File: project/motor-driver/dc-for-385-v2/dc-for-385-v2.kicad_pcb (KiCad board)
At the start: 2 copper layers, 51 x 25 mm, 44 parts, among them J1 Power, J2 Output, J3 Input, Q1 TPH11006NL, Q2 TPH11006NL, Q3 TPH11006NL, Q4 TPH11006NL, U1 IR2302, U2 IR2302, U3 L7808

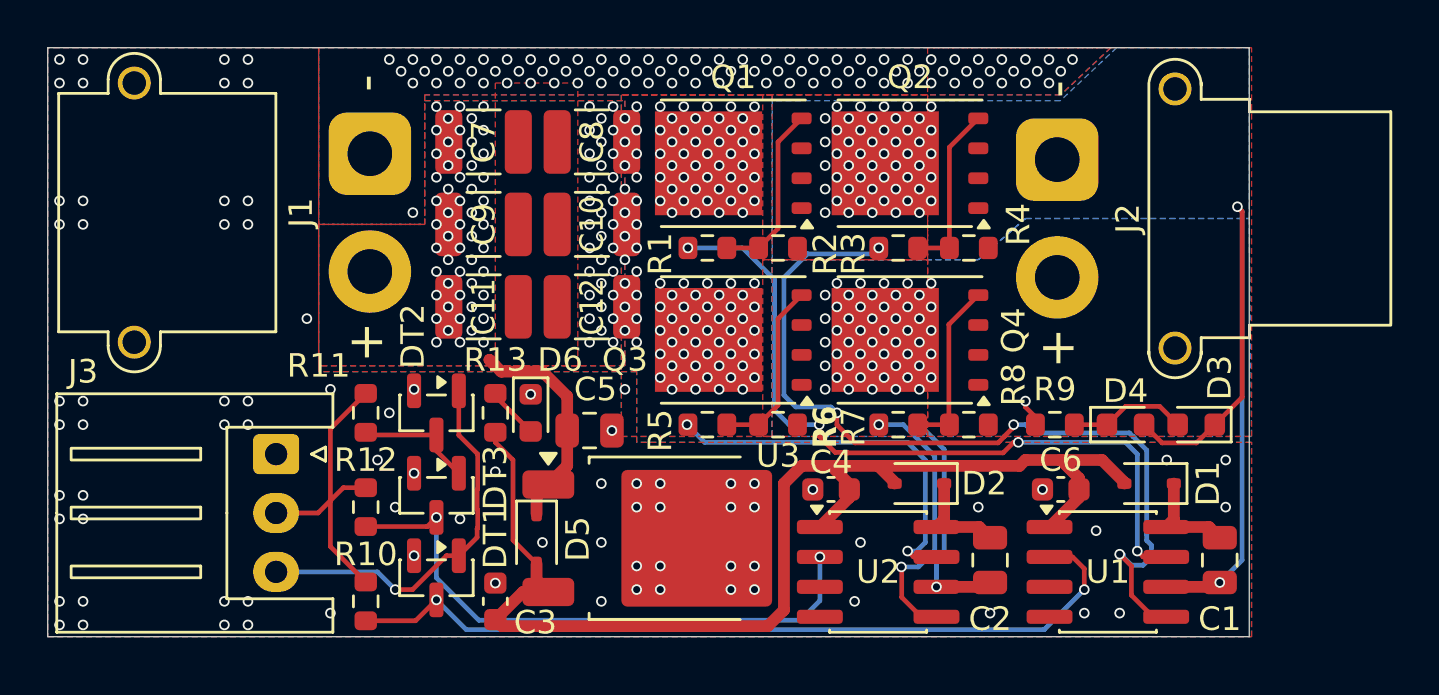
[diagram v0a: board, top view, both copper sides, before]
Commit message: 2026/07/07/11:00
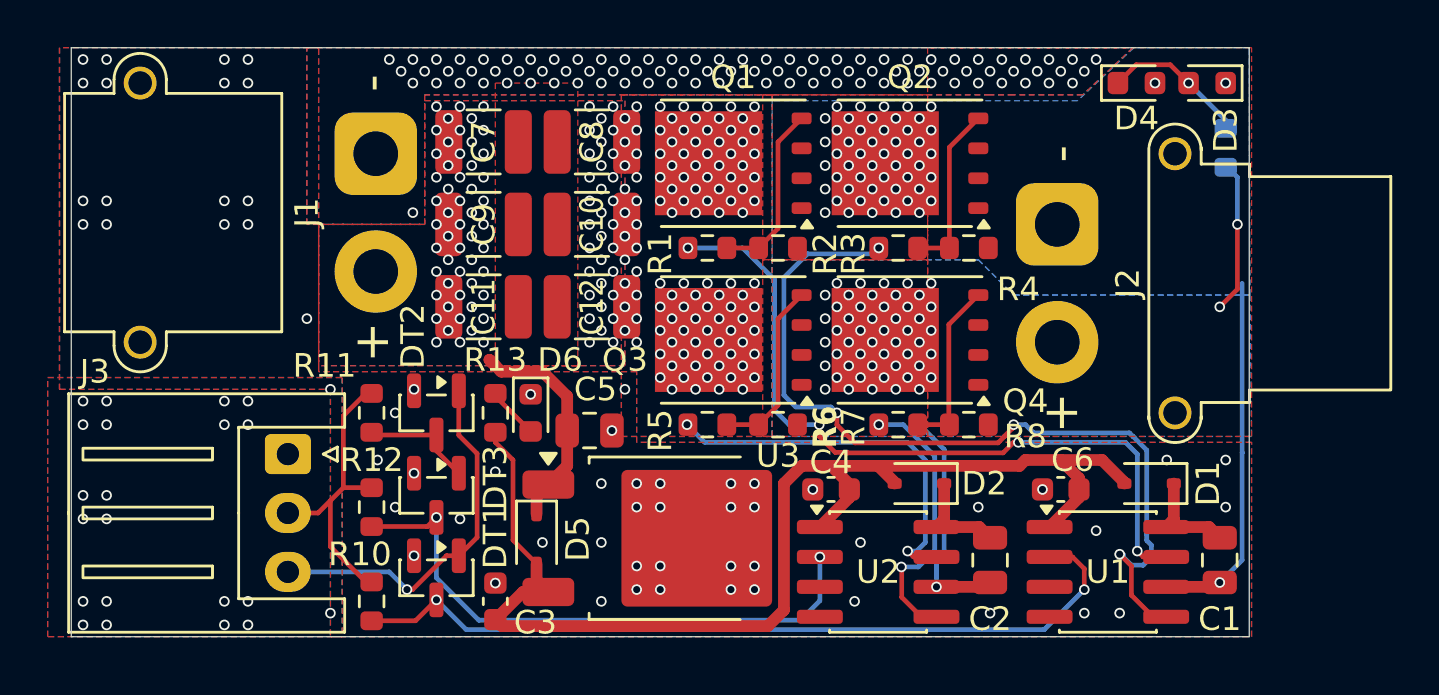
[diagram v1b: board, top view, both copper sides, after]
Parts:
- R9: moved to B.Cu
- moved D3 14.5 mm to (169.2, 61.5)
- moved D4 14.5 mm to (166.2, 61.5)
- moved R9 13.8 mm to (170.0, 64.2), turned to -90 degrees
- moved J2 2.75 mm to (162.8, 67.5)
- moved J3 0.50 mm to (130.2, 77.2)
- moved J1 0.25 mm to (133.9, 64.5)
- moved R10 0.25 mm to (133.8, 83.5)
- moved R11 0.25 mm to (133.8, 75.5)
- moved R12 0.25 mm to (133.8, 79.5)
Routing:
- net MOTOR_A: track 32.2 -> 15.4 mm, vias 52 -> 53
- net MOTOR_B: track 11.0 -> 16.3 mm, vias 52 -> 53
- net Net-(D3-A): track 5.04 -> 6.22 mm, vias 0 -> 1
- net DIR: track 16.3 -> 15.8 mm
- net PWM: track 13.5 -> 13.0 mm
- net GND: vias 171 -> 174
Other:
- board size 51 x 25 mm -> 50 x 25 mm
- board text added: "v1.0.2 @netetra07"
- board text removed: "v1.0.1 @netetra07"
